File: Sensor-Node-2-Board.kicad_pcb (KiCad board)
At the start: 2 copper layers, 100 x 100 mm, 67 parts, among them J401 EBWA-02-B, J701 PS0519, J702 EBWA-02-B, Q101 BC549, Q401 Si4944DY, SW501 SW_HELP, U201 LM393, U601 Photon 2, U701 L7805

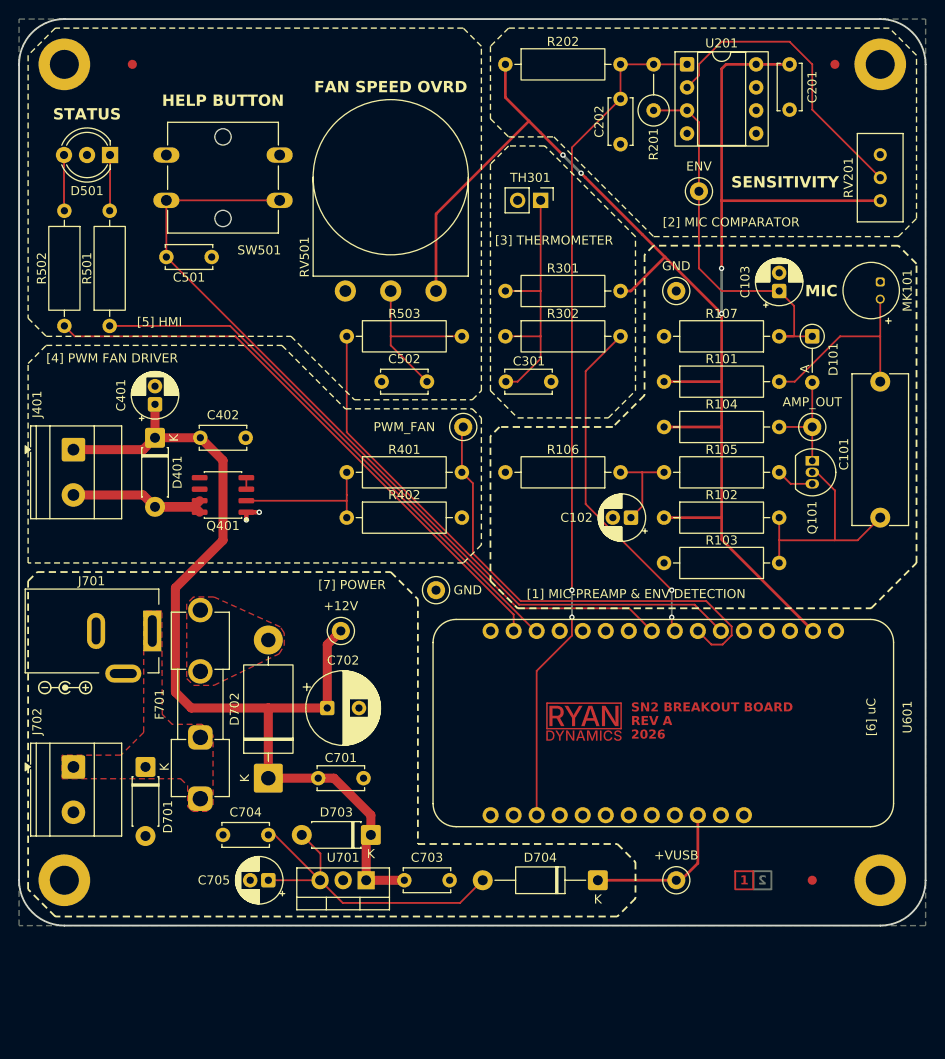
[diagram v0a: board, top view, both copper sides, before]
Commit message: feat: release
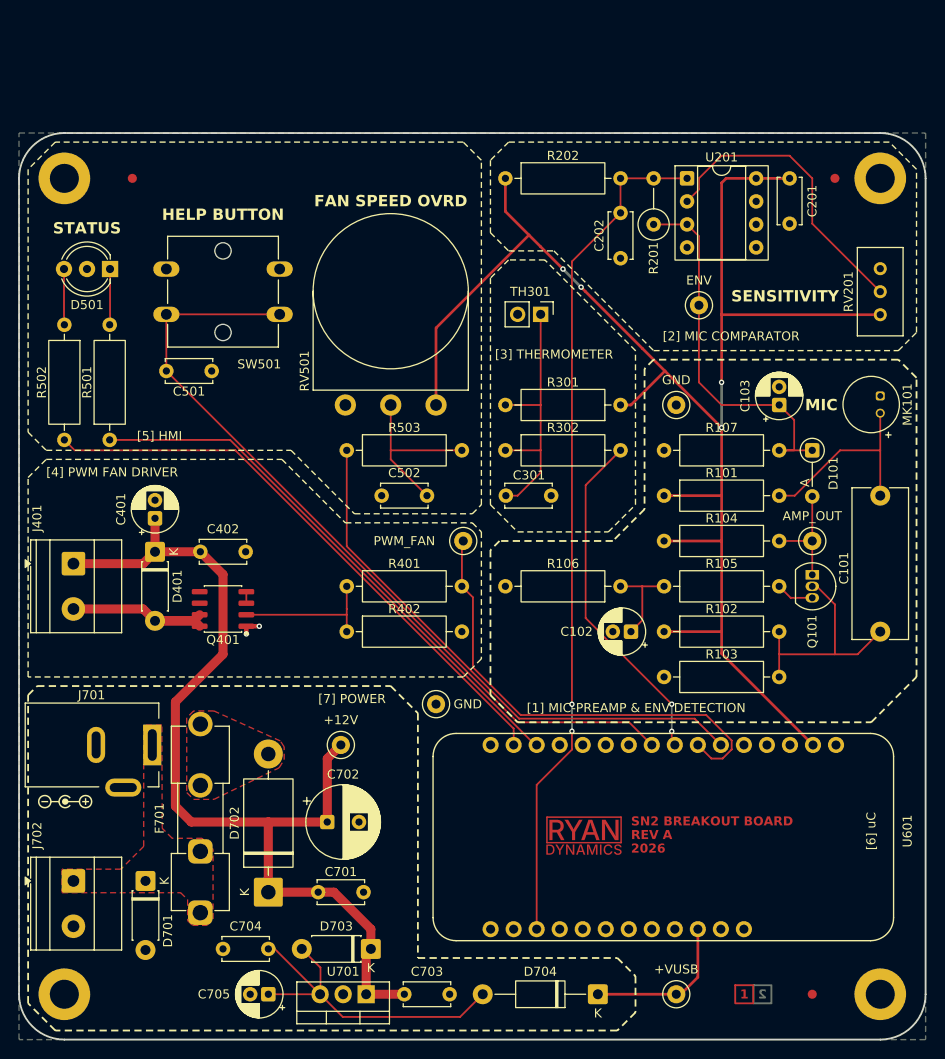
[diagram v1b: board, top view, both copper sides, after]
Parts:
- moved C701 12.6 mm to (203.0, 168.7)
- moved D702 12.6 mm to (192.5, 168.7)
- moved C101 12.6 mm to (260.0, 125.0)
- moved C102 12.6 mm to (232.5, 140.0)
- moved C103 12.6 mm to (248.8, 115.0)
- moved C201 12.6 mm to (250.0, 90.0)
- moved C202 12.6 mm to (231.3, 93.8)
- moved C301 12.6 mm to (218.7, 125.0)
- moved C401 12.6 mm to (180.0, 127.5)
- moved C402 12.6 mm to (185.0, 131.2)
- moved C501 12.6 mm to (181.2, 111.2)
- moved C502 12.6 mm to (205.0, 125.0)
- moved D101 12.6 mm to (252.5, 120.0)
- moved D401 12.6 mm to (180.0, 131.2)
- moved D501 12.6 mm to (175.0, 100.0)
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
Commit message: Update Outputs (release)
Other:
- board text added: "0.02mm"
- board text added: "0.035mm (1.00oz)"
- board text added: "1.49mm"
- board text added: "B.Mask"
- board text added: "B.Paste"
- board text added: "B.Silkscreen"
- board text added: "Copper"
- board text added: "Core"
- board text added: "Dielectric"
- board text added: "Direct Printing"
- board text added: "F.Mask"
- board text added: "F.Paste"
- board text added: "F.Silkscreen"
- board text added: "FR4_7628"
- board text added: "GBR"
- board text added: "Gerber"
- board text added: "L1 (Sig, PWR)"
- board text added: "L2 (Sig, GND)"
- board text added: "Layer"
- board text added: "Legend"
- board text added: "Material"
- board text added: "Note: external layer thicknesses are specified after plating"
- board text added: "Paste Mask"
- board text added: "Signal"
- board text added: "Solder Mask"
- board text added: "Solder Resist"
- board text added: "Thickness"
- board text added: "Total thickness: 1.6mm"
- board text added: "Type"
